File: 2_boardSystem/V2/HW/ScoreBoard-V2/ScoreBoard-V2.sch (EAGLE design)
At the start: 43 parts, among them M1 VNH5019, M2 VNH5019, M3 VNH5019, M4 VNH5019, M5 VNH5019, M6 VNH5019, U1 TXB0108

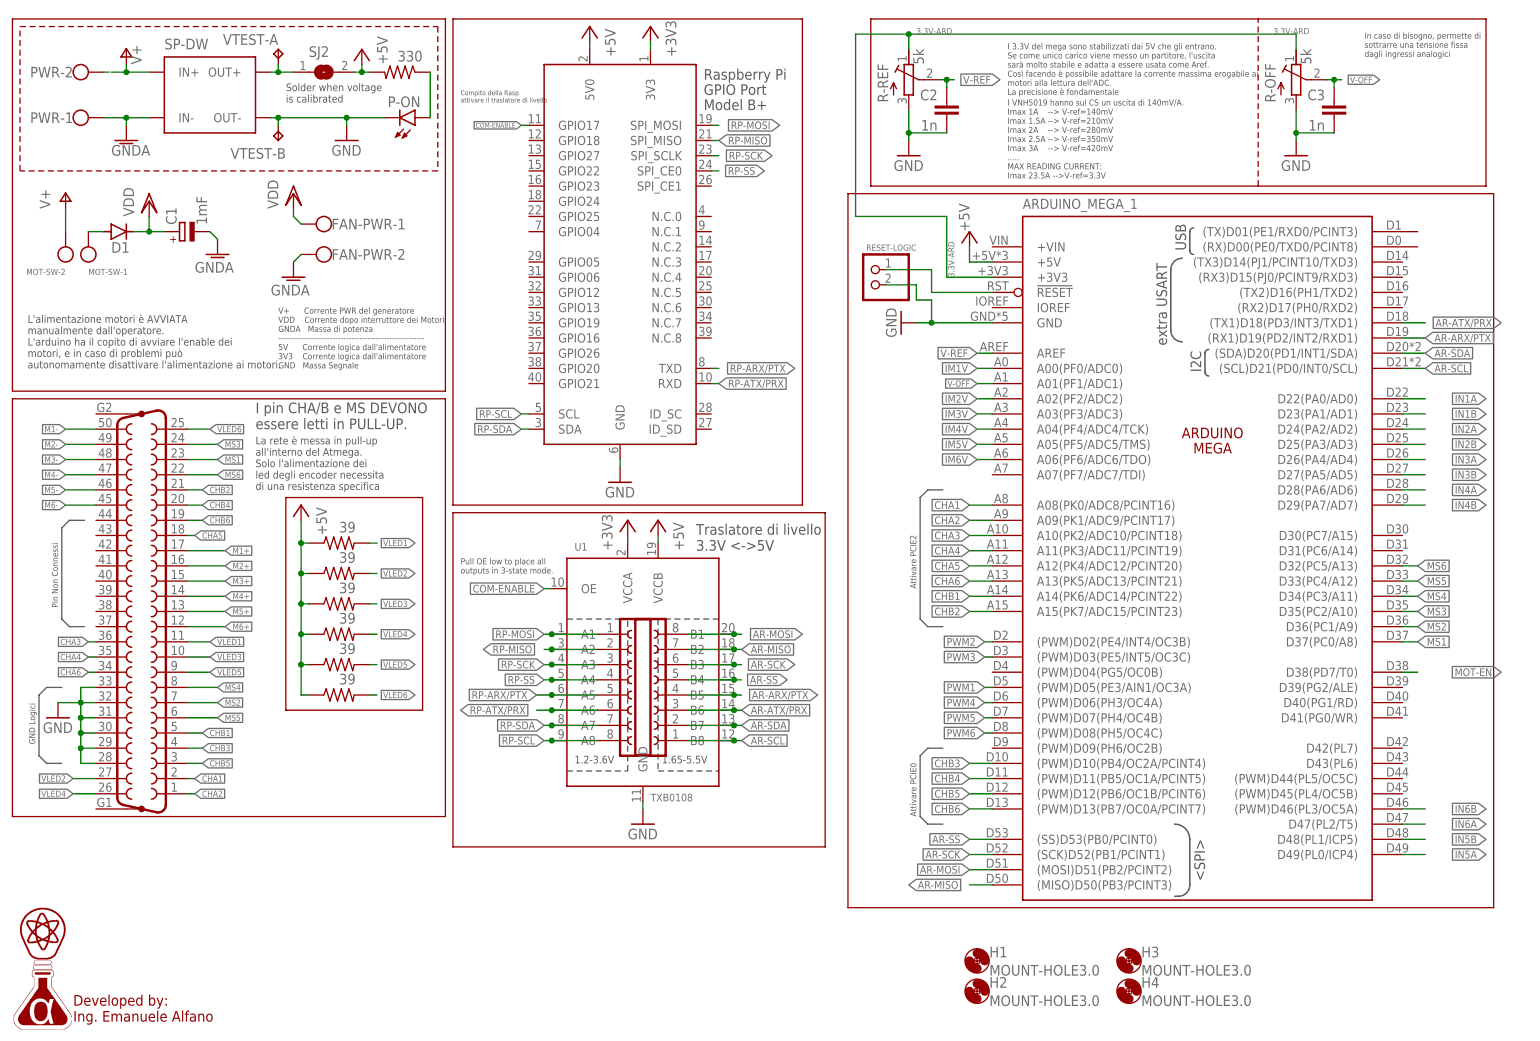
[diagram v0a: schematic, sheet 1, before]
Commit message: license and library
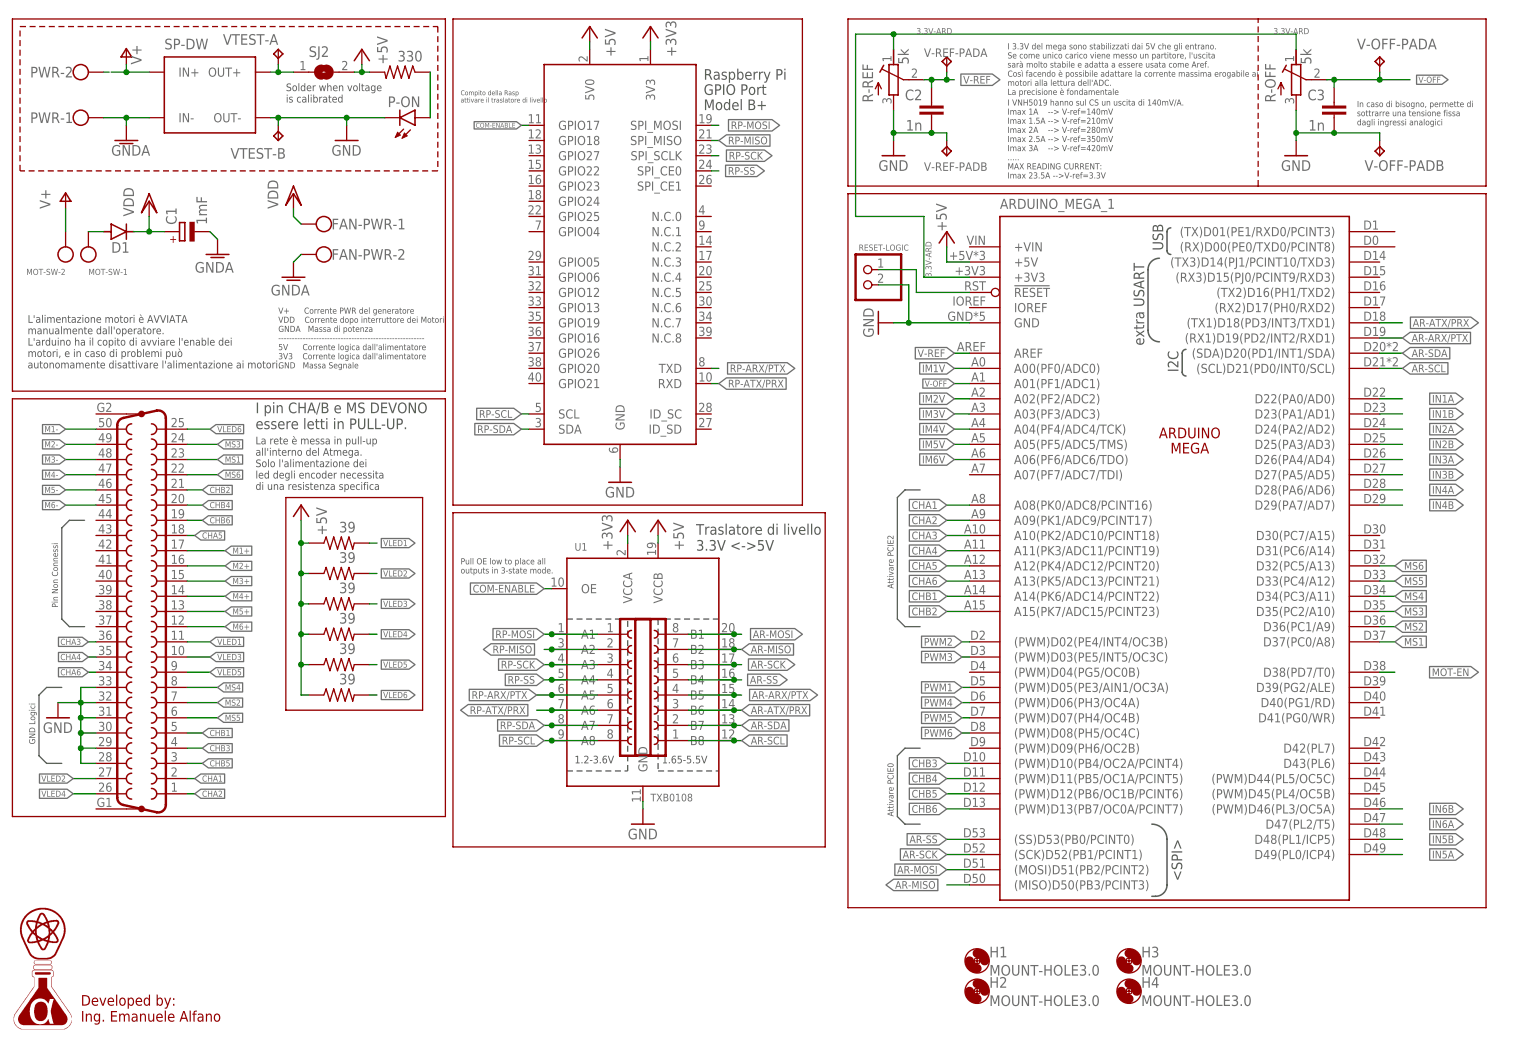
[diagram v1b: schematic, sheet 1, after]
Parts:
- added V-OFF-PAD, V-REF-PAD: TP2P2-38-17, testpad:TP2P2-38-17
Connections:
- net GND: now also V-OFF-PADB.TP, V-REF-PADB.TP
- net V-OFF: now also V-OFF-PADA.TP
- net V-REF: now also V-REF-PADA.TP
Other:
- moved on the sheet: ARDUINO_MEGA_1, C2, R-REF, RESET-LOGIC
